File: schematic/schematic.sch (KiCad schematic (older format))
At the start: 9 parts

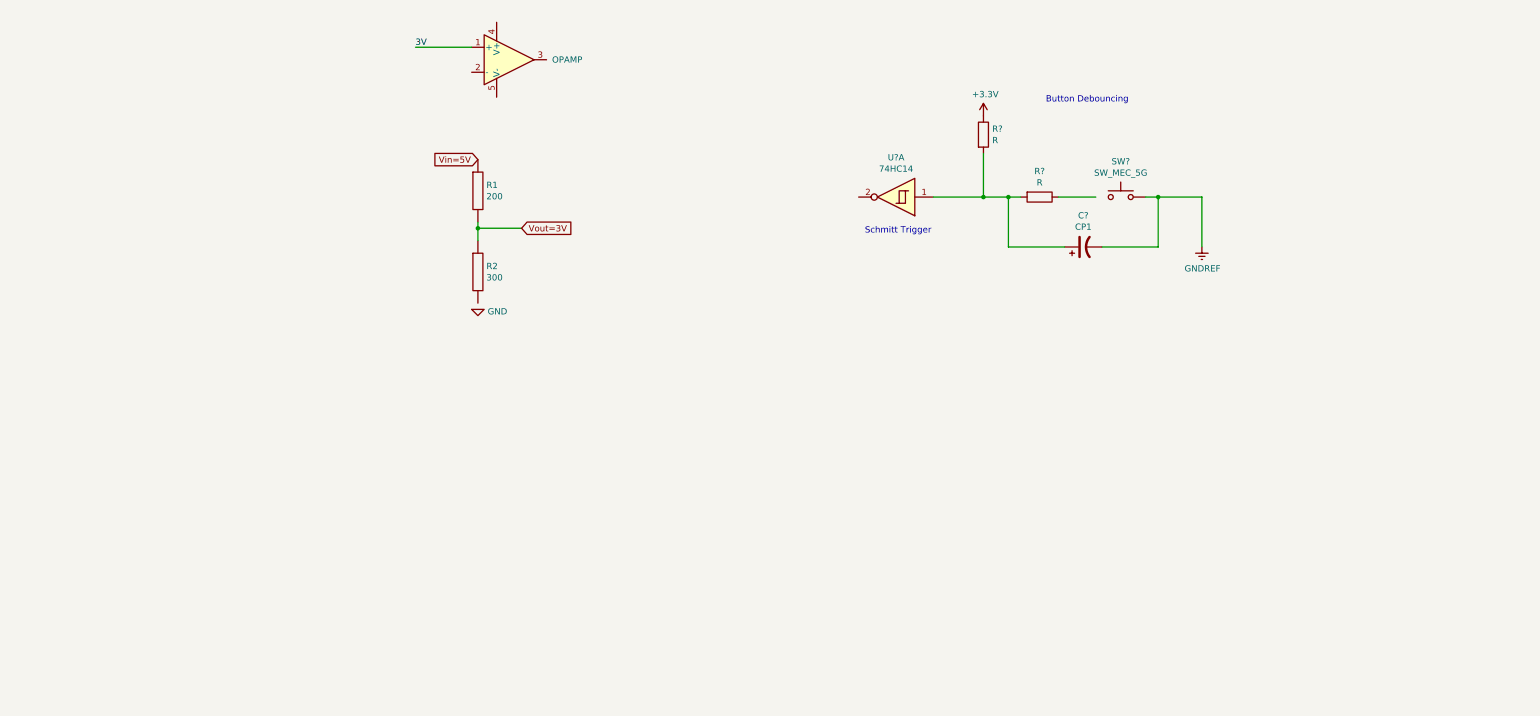
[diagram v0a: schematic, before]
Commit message: PCB started
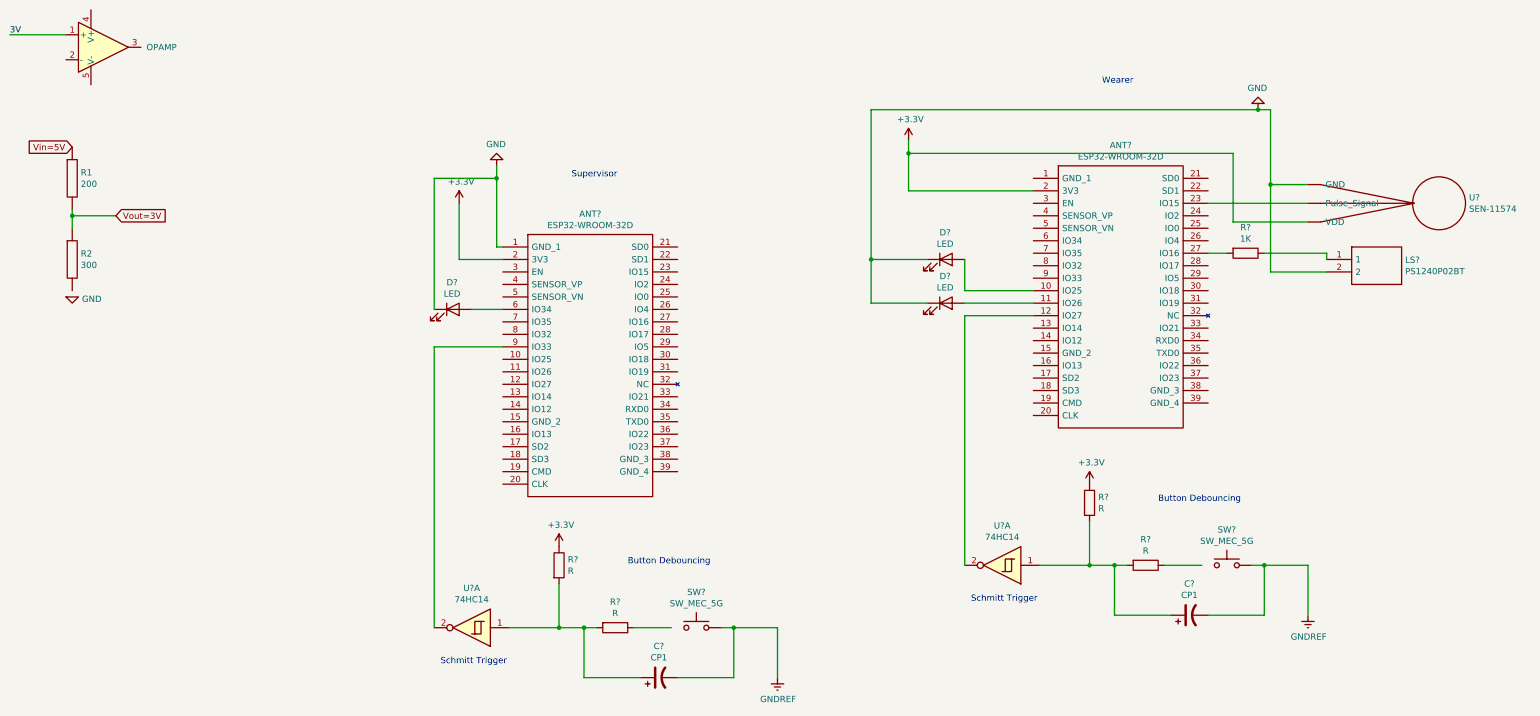
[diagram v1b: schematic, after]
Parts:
- removed C?: CP1, symbol Device:CP1
- removed R? (x2): R, symbol Device:R
- removed SW?: SW_MEC_5G, symbol Switch:SW_MEC_5G
- removed U?: 74HC14, symbol 74xx:74HC14
- added ANT? (x2): ESP32-WROOM-32D, ESP32WROOM32D, symbol Noggin:ESP32-WROOM-32D
- added C? (x2): CP1, symbol Device:CP1
- added D? (x3): LED, symbol Device:LED
- added LS?: PS1240P02BT, PS1240P02BT, symbol Noggin:PS1240P02BT
- added R? (x4): R, symbol Device:R
- added R?: 1K, symbol Device:R
- added SW? (x2): SW_MEC_5G, symbol Switch:SW_MEC_5G
- added U?: SEN-11574, symbol Noggin:SEN-11574
- added U? (x2): 74HC14, symbol 74xx:74HC14
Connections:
- net +3V3: now also ANT?.2 (3V3), ANT?.2 (3V3), R?.1, R?.1, U?.~ (VDD)
- net GNDREF: now also C?.2, C?.2, SW?.3 (B), SW?.3 (B), SW?.4 (B), SW?.4 (B)
- new net: ANT?.10 (IO25), D?.2 (A)
- new net: ANT?.11 (IO26), D?.2 (A)
- new net: ANT?.12 (IO27), U?.2
- new net: ANT?.23 (IO15), U?.~ (VDD)
- new net: ANT?.27 (IO16), R?.2
- new net: C?.1, R?.2, R?.2, U?.1 (x2)
- new net: R?.1, SW?.1 (A), SW?.2 (A) (x2)
- new net: LS?.1, R?.1
- new net: ANT?.6 (IO34), D?.2 (A)
- new net: ANT?.9 (IO33), U?.2
- new net GND: ANT?.1 (GND_1), D?.1 (K), D?.1 (K), D?.1 (K), LS?.2, U?.~ (VDD)
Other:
- note added: "Supervisor\n"
- note added: "Wearer\n"
- moved on the sheet: R1, R2
